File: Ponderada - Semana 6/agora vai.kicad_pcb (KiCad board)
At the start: 2 copper layers, 8 parts, among them J1 Alimentacao, J2 Conn_01x02_Pin, Q1 BC108

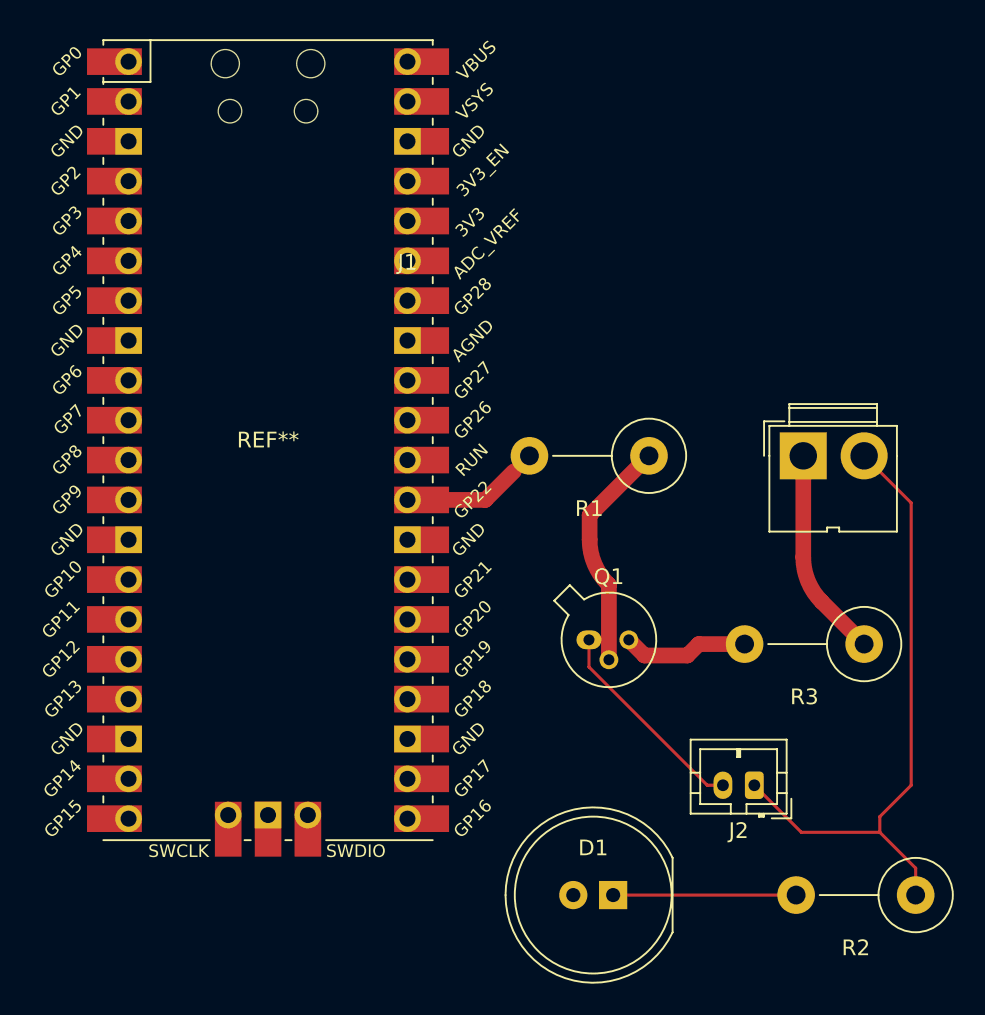
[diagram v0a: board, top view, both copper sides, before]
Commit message: ponderada - semana 6
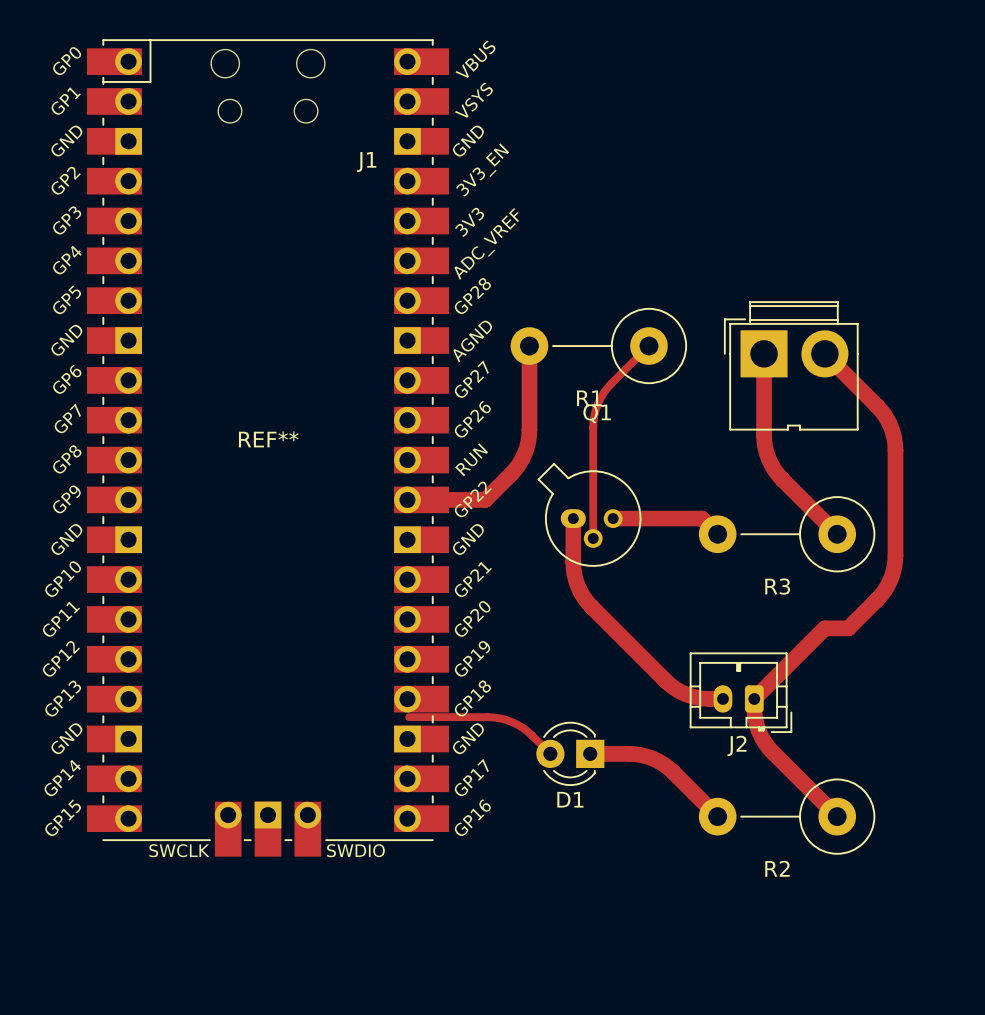
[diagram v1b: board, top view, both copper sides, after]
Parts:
- D1: footprint LED_THT:LED_D10.0mm -> LED_THT:LED_D3.0mm
- moved D1 9.12 mm to (131.5, 119.0)
- moved Q1 7.79 mm to (130.5, 104.0)
- moved R3 7.21 mm to (147.3, 105.0)
- moved R2 7.07 mm to (147.3, 123.0)
- moved R1 7.00 mm to (135.3, 93.0)
- moved J1 6.96 mm to (142.6, 93.5)
- moved J2 5.50 mm to (142.0, 115.5)
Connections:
- J2 pad 2: Net-(J2-Pin_2) -> Net-(Q1-B)
- Q1 pad 1: Net-(J2-Pin_2) -> Net-(Q1-B)
- REF** pad 24: (no net) -> Net-(D1-A)
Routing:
- net Net-(Q1-B): track 14.9 -> 30.1 mm
- net Net-(J2-Pin_2): track 13.4 -> 0.00 mm
- net Net-(D1-A): track 0.00 -> 12.3 mm
- net Net-(U1-GPIO22): track 10.0 -> 18.2 mm
- net GND: track 40.3 -> 37.6 mm
- net Net-(D1-K): track 11.7 -> 9.59 mm
- net Net-(Q1-C): track 8.10 -> 7.08 mm
